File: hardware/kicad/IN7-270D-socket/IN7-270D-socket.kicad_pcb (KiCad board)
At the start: 2 copper layers, 31.8 x 31.8 mm, 5 parts, among them J1 Conn_01x08_Pin, J2 Conn_01x08_Pin, T1 IN-7

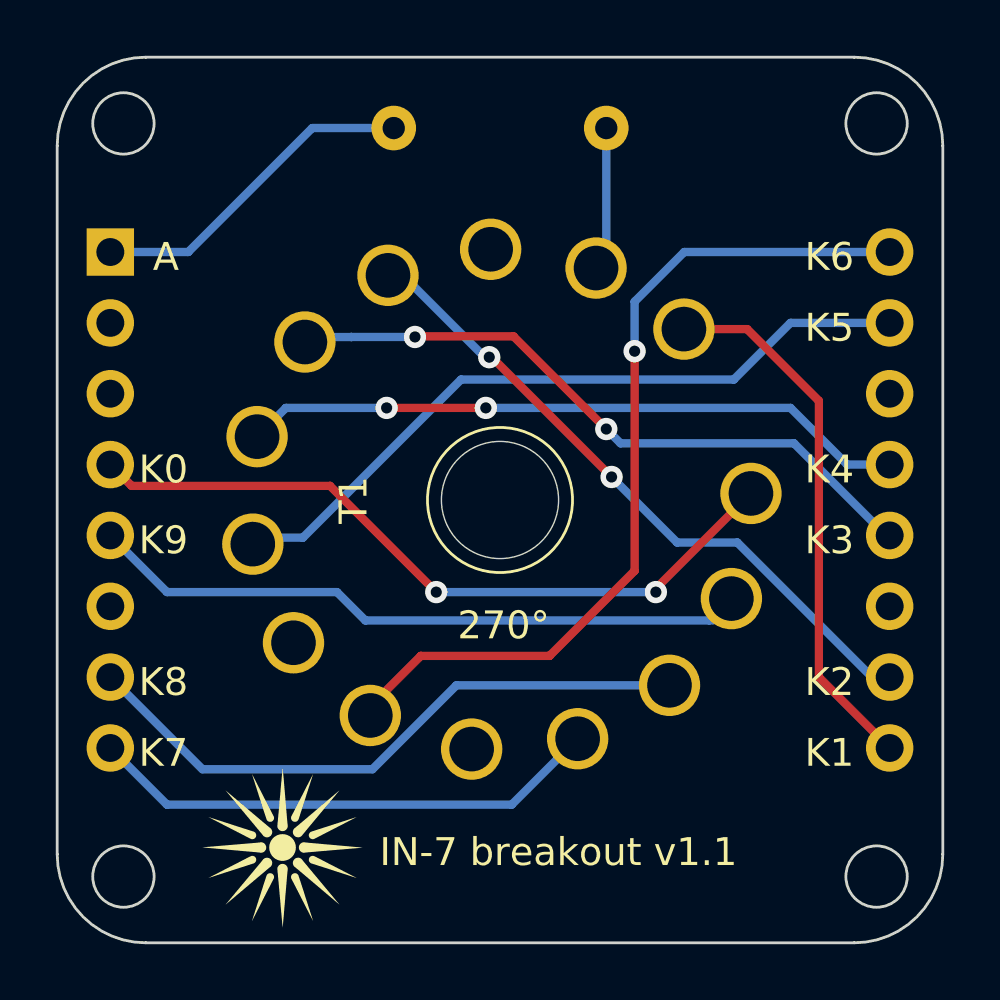
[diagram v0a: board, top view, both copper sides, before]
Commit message: bowen minor updates
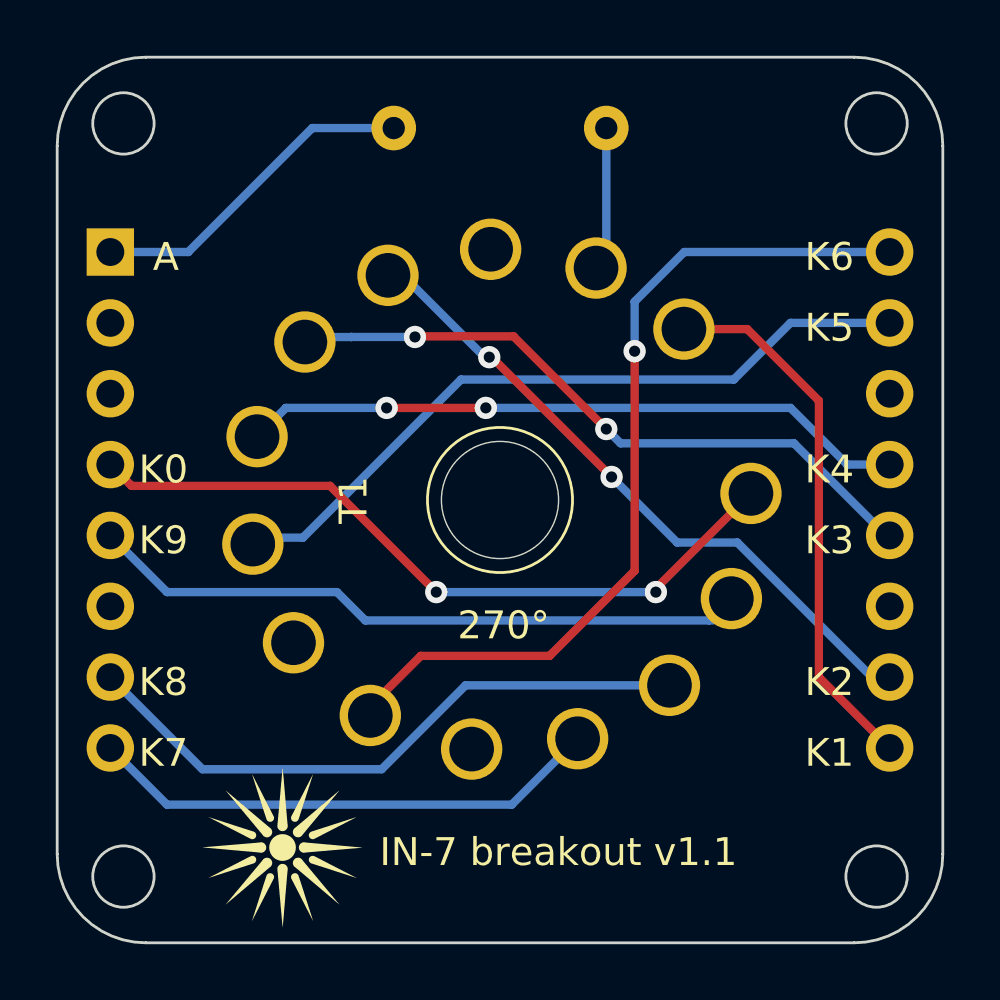
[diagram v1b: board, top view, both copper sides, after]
